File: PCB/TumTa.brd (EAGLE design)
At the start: 100 x 80 mm, 20 parts

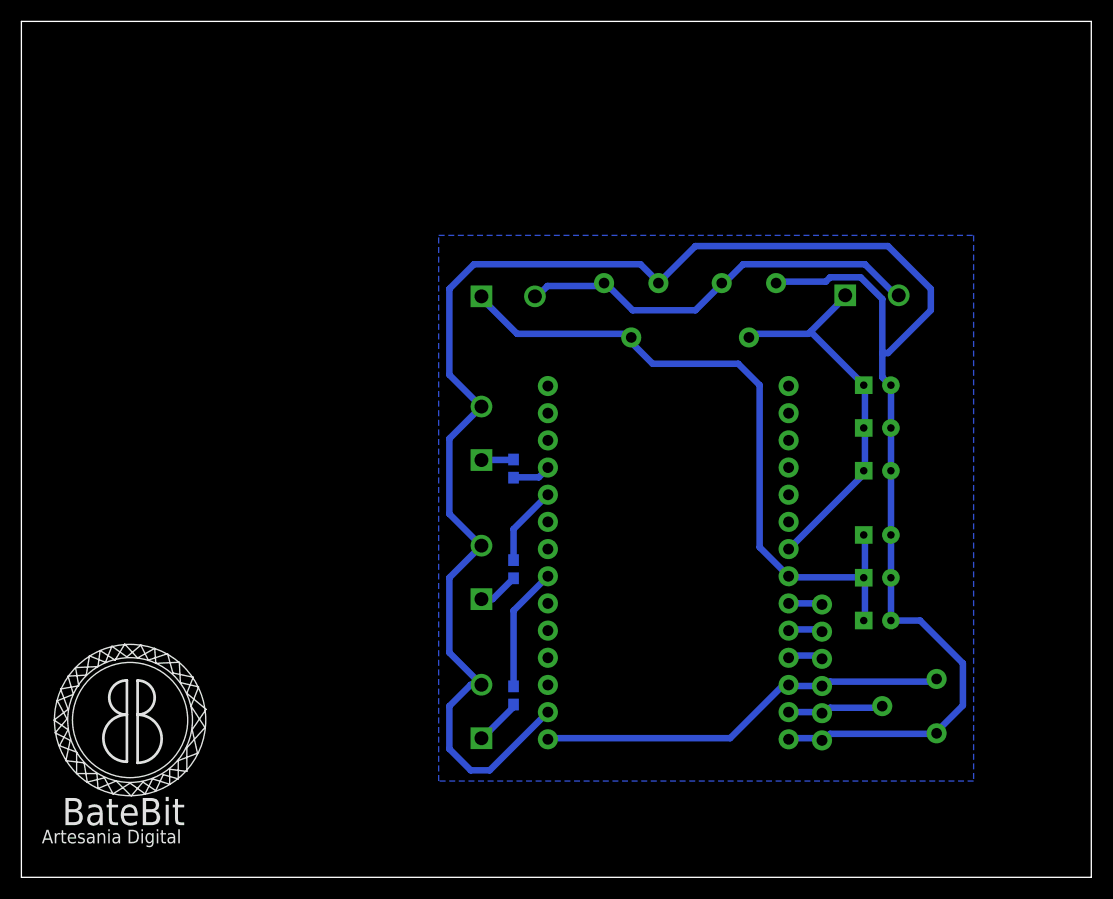
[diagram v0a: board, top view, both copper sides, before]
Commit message: v0_2_9
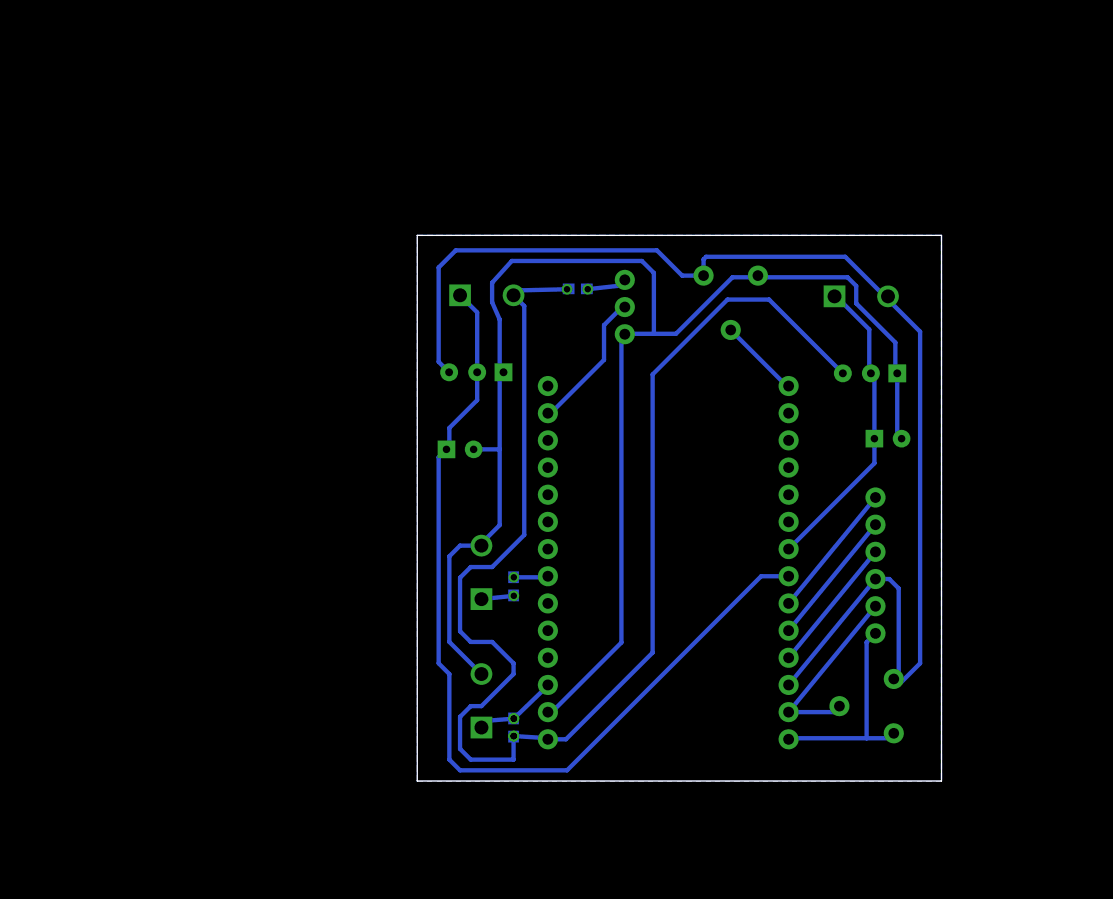
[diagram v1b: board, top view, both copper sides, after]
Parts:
- removed C1, C2, C3, C4, C5, C6: (no value), SparkFun-Passives:CPOL-RADIAL-10UF-25V
- removed FL1: FRAME-LETTER_BATEBIT, SparkFun-Retired:BATEBIT
- removed JP1: (no value), SparkFun-Connectors:1X06
- removed LED1(VERDE): SCREWTERMINAL-25MM, SparkFun-Connectors:SCREWTERMINAL-5MM-2
- removed R1: 100, SparkFun-Resistors:0603-RES
- added C_TA, C_TUM: (no value), SparkFun-Passives:CPOL-RADIAL-10UF-25V
- added FTDI: (no value), SparkFun-Connectors:1X06
- added MODO: (no value), SparkFun-Electromechanical:SWITCH-SPDT
- added R5: 4.7K, SparkFun-Resistors:0603-RES
- added THRESHOLD: (no value), SparkFun-Electromechanical:TRIM_POT_BR
- TA_CALIB, TUM_CALIB: value (none) -> TRIMPOT_MULTIVOLTAS; device SparkFun-Electromechanical:TRIM_POT_BR -> SparkFun-Electromechanical:TRIMPOT_MULTIVOLTAS
- moved TA 36.0 mm to (41.0, 54.4)
- moved TUM 33.0 mm to (76.0, 54.3)
- moved TUM_CALIB 28.2 mm to (84.1, 45.1)
- moved TA_CALIB 22.1 mm to (47.3, 45.2)
- moved LED2(AMARELO) 13.0 mm to (43.0, 26.0)
- moved R2 11.0 mm to (46.0, 27.2), turned to 90 degrees
- moved AREF 4.00 mm to (79.0, 16.0)
- moved R4 3.00 mm to (46.0, 14.0), turned to 270 degrees
- moved SWITCH_STANDBY 1.00 mm to (43.0, 14.0)
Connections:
- removed net 3.3V: TA.2, TA_CALIB.3, TUM.2, TUM_CALIB.3
- removed net D6: FIO_SHIELD.7, R4.2
- removed net D9: FIO_SHIELD.10, R1.2
- new net N$1: FIO_SHIELD.28, THRESHOLD.2
- new net N$4: MODO.3, R5.2
- net 3V3: now also FTDI.4, R4.2, R5.1, TA.2, TA_CALIB.3, THRESHOLD.3, TUM.2, TUM_CALIB.3; no longer JP1.4
- net A0: now also C_TUM.1, FIO_SHIELD.22; no longer C1.1, C2.1, C3.1, FIO_SHIELD.21
- net A1: now also C_TA.1, FIO_SHIELD.21; no longer C4.1, C5.1, C6.1, FIO_SHIELD.22
- net AREF: now also FTDI.5; no longer JP1.5
- net D10: now also FIO_SHIELD.7; no longer FIO_SHIELD.11
- net DTR: now also FTDI.1; no longer JP1.1
- net GND: now also C_TA.2, C_TUM.2, FTDI.6, MODO.1, THRESHOLD.1; no longer C1.2, C2.2, C3.2, C4.2, C5.2, C6.2, JP1.6, LED1(VERDE).2
- net N$2: now also FIO_SHIELD.3
- net N$3: now also FIO_SHIELD.13, MODO.2; no longer LED1(VERDE).1, R1.1
- net RXI: now also FTDI.3; no longer JP1.3
- net TXO: now also FTDI.2; no longer JP1.2
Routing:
- net 3V3: track 39.0 -> 251.5 mm, vias 0 -> 3
- net A1: track 36.2 -> 85.6 mm
- net 3.3V: track 38.9 -> 0.00 mm
- net A0: track 64.1 -> 28.6 mm
- net GND: track 193.7 -> 166.1 mm
- net D6: track 11.6 -> 0.00 mm
- net DTR: track 3.18 -> 12.8 mm
- net TXO: track 3.30 -> 12.8 mm
- net N$3: track 3.81 -> 13.2 mm
- net RXI: track 3.46 -> 12.8 mm
- net AREF: track 9.02 -> 17.8 mm
- net N$1: track 0.00 -> 7.58 mm
- net D9: track 7.44 -> 0.00 mm
- net N$4: track 0.00 -> 3.78 mm, vias 0 -> 1
- net N$2: track 4.61 -> 7.90 mm, vias 0 -> 2
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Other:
- board size 100 x 80 mm -> 49 x 51 mm
- board text added: "BLK"
- board text added: "GRN"
